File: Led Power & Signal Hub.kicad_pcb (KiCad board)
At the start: 2 copper layers, 3 parts, among them J1 Conn_01x03_Female, J2 Conn_01x04_Female, J3 Conn_01x03_Female

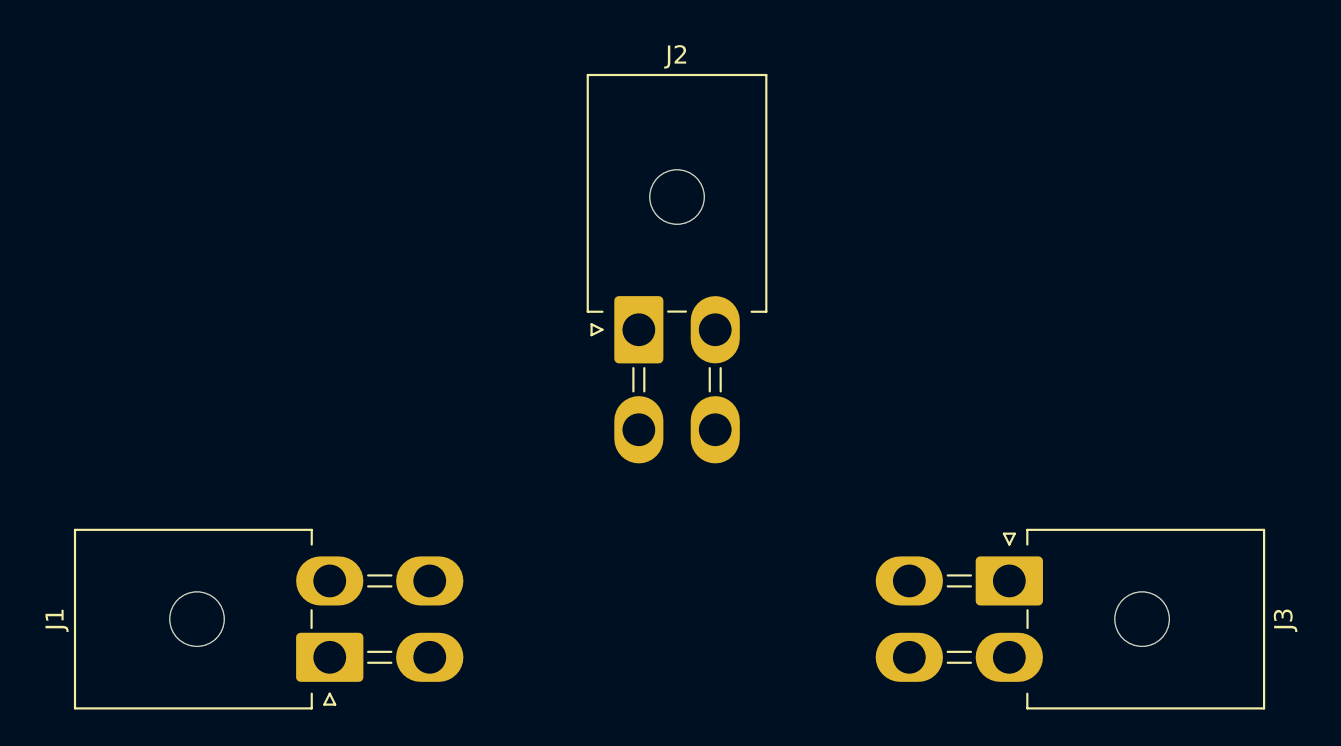
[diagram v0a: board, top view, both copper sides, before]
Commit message: Gotowe PCB
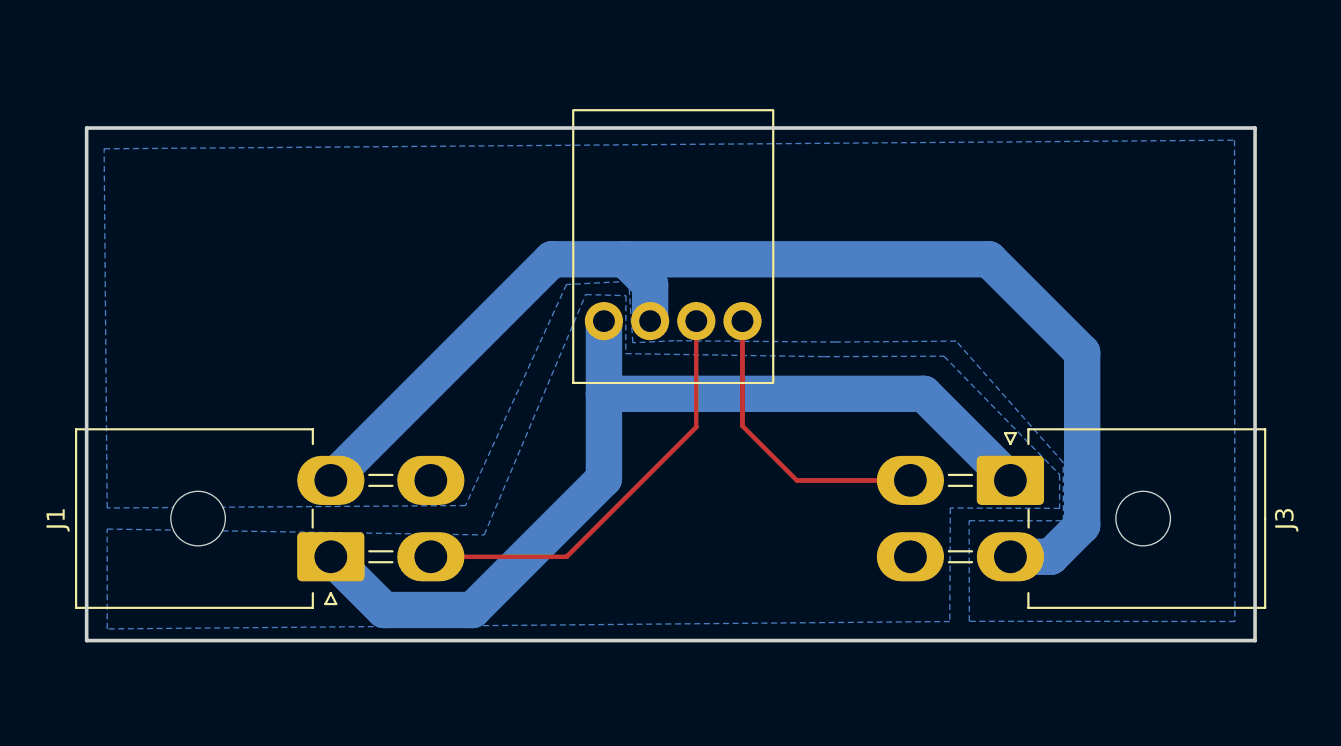
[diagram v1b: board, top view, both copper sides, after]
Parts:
- J2: footprint Connector_Molex:Molex_Mini-Fit_Jr_5569-04A2_2x02_P4.20mm_Horizontal -> SamacSys_Parts:Gniazdo WF kątowe
- moved J1 5.53 mm to (103.8, 96.2)
- moved J3 5.53 mm to (141.1, 92.0)
- moved J2 1.97 mm to (118.8, 83.3)
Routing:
- net Net-(J1-Pad2): track 0.00 -> 66.6 mm
- net Net-(J1-Pad1): track 0.00 -> 52.2 mm
- net Net-(J1-Pad3): track 0.00 -> 23.4 mm
- net Net-(J2-Pad4): track 0.00 -> 16.2 mm
- added copper zone on B.Cu, net Net-(J1-Pad1)
- added copper zone on B.Cu, net Net-(J1-Pad2)
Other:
- board outline added: 64.3 x 28.2 mm
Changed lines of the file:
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@@
   )
   (setup
+    (stackup
+      (layer "F.SilkS" (type "Top Silk Screen"))
+      (layer "F.Paste" (type "Top Solder Paste"))
+      (layer "F.Mask" (type "Top Solder Mask") (thickness 0.01))
+      (layer "F.Cu" (type "copper") (thickness 0.035))
+      (layer "dielectric 1" (type "core") (thickness 1.51) (material "FR4") (epsilon_r 4.5) (loss_tangent 0.02))
+      (layer "B.Cu" (type "copper") (thickness 0.035))
+      (layer "B.Mask" (type "Bottom Solder Mask") (thickness 0.01))
+      (layer "B.Paste" (type "Bottom Solder Paste"))
+      (layer "B.SilkS" (type "Bottom Silk Screen"))
+      (copper_finish "None")
+      (dielectric_constraints no)
+    )
     (pad_to_mask_clearance 0)
     (pcbplotparams
@@
   (net 3 "Net-(J1-Pad3)")
   (net 4 "Net-(J2-Pad4)")
-  (footprint "Connector_Molex:Molex_Mini-Fit_Jr_5569-04A2_2x02_P4.20mm_Horizontal" (layer "F.Cu")
-    (at 120.7 83.765)
-    (descr "Molex Mini-Fit Jr. Power Connectors, old mpn/engineering number: 5569-04A2, example for new mpn: 39-30-0040, 2 Pins per row, Mounting: Snap-in Plastic Peg PCB Lock (http://www.molex.com/pdm_docs/sd/039300020_sd.pdf), generated with kicad-footprint-generator")
-    (tags "connector Molex Mini-Fit_Jr top entryplastic_peg")
+  (footprint "SamacSys_Parts:Gniazdo WF kątowe" (layer "F.Cu")
+    (at 118.79 83.29)
     (property "Sheetfile" "Led Power & Signal Hub.kicad_sch")
     (property "Sheetname" "")
     (attr through_hole)
-    (fp_text reference "J2" (at 2.1 -15.1) (layer "F.SilkS")
-      (effects (font (size 1 1) (thickness 0.15)))
-    )
-    (fp_text value "Conn_01x04_Female" (at 2.1 8.55) (layer "F.Fab")
-      (effects (font (size 1 1) (thickness 0.15)))
-    )
-    (fp_text user "${REFERENCE}" (at 2.1 -13.2) (layer "F.Fab")
-      (effects (font (size 1 1) (thickness 0.15)))
-    )
-    (fp_line (start -2 0) (end -2.6 0.3) (layer "F.SilkS") (width 0.12))
-    (fp_line (start -2 -0.99) (end -2.81 -0.99) (layer "F.SilkS") (width 0.12))
-    (fp_line (start 7.01 -14.01) (end 2.1 -14.01) (layer "F.SilkS") (width 0.12))
-    (fp_line (start 1.61 -1) (end 2.59 -1) (layer "F.SilkS") (width 0.12))
-    (fp_line (start 3.9 2.11) (end 3.9 3.39) (layer "F.SilkS") (width 0.12))
-    (fp_line (start -2.81 -14.01) (end 2.1 -14.01) (layer "F.SilkS") (width 0.12))
-    (fp_line (start -2.81 -0.99) (end -2.81 -14.01) (layer "F.SilkS") (width 0.12))
-    (fp_line (start -2.6 0.3) (end -2.6 -0.3) (layer "F.SilkS") (width 0.12))
-    (fp_line (start -2.6 -0.3) (end -2 0) (layer "F.SilkS") (width 0.12))
-    (fp_line (start 4.5 2.11) (end 4.5 3.39) (layer "F.SilkS") (width 0.12))
-    (fp_line (start -0.3 2.11) (end -0.3 3.39) (layer "F.SilkS") (width 0.12))
-    (fp_line (start 0.3 2.11) (end 0.3 3.39) (layer "F.SilkS") (width 0.12))
-    (fp_line (start 7.01 -0.99) (end 7.01 -14.01) (layer "F.SilkS") (width 0.12))
-    (fp_line (start 6.2 -0.99) (end 7.01 -0.99) (layer "F.SilkS") (width 0.12))
-    (fp_line (start -3.2 -14.4) (end -3.2 7.85) (layer "F.CrtYd") (width 0.05))
-    (fp_line (start 7.4 -14.4) (end -3.2 -14.4) (layer "F.CrtYd") (width 0.05))
-    (fp_line (start 7.4 7.85) (end 7.4 -14.4) (layer "F.CrtYd") (width 0.05))
-    (fp_line (start -3.2 7.85) (end 7.4 7.85) (layer "F.CrtYd") (width 0.05))
-    (fp_line (start -1 -1.1) (end 0 -2.514214) (layer "F.Fab") (width 0.1))
-    (fp_line (start -2.7 -13.9) (end -2.7 -1.1) (layer "F.Fab") (width 0.1))
-    (fp_line (start -2.7 -1.1) (end 6.9 -1.1) (layer "F.Fab") (width 0.1))
-    (fp_line (start 0 -2.514214) (end 1 -1.1) (layer "F.Fab") (width 0.1))
-    (fp_line (start 6.9 -1.1) (end 6.9 -13.9) (layer "F.Fab") (width 0.1))
-    (fp_line (start 6.9 -13.9) (end -2.7 -13.9) (layer "F.Fab") (width 0.1))
-    (pad "" np_thru_hole circle (at 2.1 -7.3) (size 3 3) (drill 3) (layers *.Cu *.Mask))
-    (pad "1" thru_hole roundrect (at 0 0) (size 2.7 3.7) (drill 1.8) (layers *.Cu *.Mask) (roundrect_rratio 0.092593)
+    (fp_text reference "J2" (at 0 -0.5 unlocked) (layer "F.SilkS") hide
+      (effects (font (size 1 1) (thickness 0.15)))
+    )
+    (fp_text value "Conn_01x04_Female" (at 0.1 5.29 unlocked) (layer "F.Fab")
+      (effects (font (size 1 1) (thickness 0.15)))
+    )
+    (fp_text user "${REFERENCE}" (at 0.23 7.23 unlocked) (layer "F.Fab")
+      (effects (font (size 1 1) (thickness 0.15)))
+    )
+    (fp_rect (start -1.7 3.4) (end 9.3 -11.6) (layer "F.SilkS") (width 0.12) (fill none))
+    (pad "1" thru_hole circle (at -0.01 0) (size 2.1 2.1) (drill 1.2) (layers *.Cu *.Mask)
       (net 1 "Net-(J1-Pad1)") (pinfunction "Pin_1") (pintype "passive"))
-    (pad "2" thru_hole oval (at 4.2 0) (size 2.7 3.7) (drill 1.8) (layers *.Cu *.Mask)
+    (pad "2" thru_hole circle (at 2.53 0) (size 2.1 2.1) (drill 1.2) (layers *.Cu *.Mask)
       (net 2 "Net-(J1-Pad2)") (pinfunction "Pin_2") (pintype "passive"))
-    (pad "3" thru_hole oval (at 0 5.5) (size 2.7 3.7) (drill 1.8) (layers *.Cu *.Mask)
+    (pad "3" thru_hole circle (at 5.07 0) (size 2.1 2.1) (drill 1.2) (layers *.Cu *.Mask)
       (net 3 "Net-(J1-Pad3)") (pinfunction "Pin_3") (pintype "passive"))
-    (pad "4" thru_hole oval (at 4.2 5.5) (size 2.7 3.7) (drill 1.8) (layers *.Cu *.Mask)
+    (pad "4" thru_hole circle (at 7.61 0) (size 2.1 2.1) (drill 1.2) (layers *.Cu *.Mask)
       (net 4 "Net-(J2-Pad4)") (pinfunction "Pin_4") (pintype "passive"))
-    (model "${KICAD6_3DMODEL_DIR}/Connector_Molex.3dshapes/Molex_Mini-Fit_Jr_5569-04A2_2x02_P4.20mm_Horizontal.wrl"
-      (offset (xyz 0 0 0))
-      (scale (xyz 1 1 1))
-      (rotate (xyz 0 0 0))
-    )
   )
   (footprint "Connector_Molex:Molex_Mini-Fit_Jr_5569-04A2_2x02_P4.20mm_Horizontal" (layer "F.Cu")
-    (at 103.7 101.78 90)
+    (at 103.76 96.25 90)
     (descr "Molex Mini-Fit Jr. Power Connectors, old mpn/engineering number: 5569-04A2, example for new mpn: 39-30-0040, 2 Pins per row, Mounting: Snap-in Plastic Peg PCB Lock (http://www.molex.com/pdm_docs/sd/039300020_sd.pdf), generated with kicad-footprint-generator")
     (tags "connector Molex Mini-Fit_Jr top entryplastic_peg")
@@
   )
   (footprint "Connector_Molex:Molex_Mini-Fit_Jr_5569-04A2_2x02_P4.20mm_Horizontal" (layer "F.Cu")
-    (at 141.075 97.58 -90)
+    (at 141.135 92.05 -90)
     (descr "Molex Mini-Fit Jr. Power Connectors, old mpn/engineering number: 5569-04A2, example for new mpn: 39-30-0040, 2 Pins per row, Mounting: Snap-in Plastic Peg PCB Lock (http://www.molex.com/pdm_docs/sd/039300020_sd.pdf), generated with kicad-footprint-generator")
     (tags "connector Molex Mini-Fit_Jr top entryplastic_peg")
@@
     )
   )
+  (gr_rect (start 90.33 72.67) (end 154.59 100.86) (layer "Edge.Cuts") (width 0.2) (fill none))
+  (segment (start 118.78 87.29) (end 118.78 83.29) (width 2) (layer "B.Cu") (net 1))
+  (segment (start 103.76 96.25) (end 106.69 99.18) (width 2) (layer "B.Cu") (net 1))
+  (segment (start 136.375 87.29) (end 141.135 92.05) (width 2) (layer "B.Cu") (net 1))
+  (segment (start 106.69 99.18) (end 111.55 99.18) (width 2) (layer "B.Cu") (net 1))
+  (segment (start 118.78 91.95) (end 118.78 87.29) (width 2) (layer "B.Cu") (net 1))
+  (segment (start 118.78 87.29) (end 136.375 87.29) (width 2) (layer "B.Cu") (net 1))
+  (segment (start 111.55 99.18) (end 118.78 91.95) (width 2) (layer "B.Cu") (net 1))
+  (segment (start 119.93 79.89) (end 121.32 81.28) (width 2) (layer "B.Cu") (net 2))
+  (segment (start 143.35 96.25) (end 141.135 96.25) (width 2) (layer "B.Cu") (net 2))
+  (segment (start 121.32 81.28) (end 121.32 83.29) (width 2) (layer "B.Cu") (net 2))
+  (segment (start 103.76 92.05) (end 115.92 79.89) (width 2) (layer "B.Cu") (net 2))
+  (segment (start 119.93 79.89) (end 139.95 79.89) (width 2) (layer "B.Cu") (net 2))
+  (segment (start 115.92 79.89) (end 119.93 79.89) (width 2) (layer "B.Cu") (net 2))
+  (segment (start 145.08 94.52) (end 143.35 96.25) (width 2) (layer "B.Cu") (net 2))
+  (segment (start 145.08 85.02) (end 145.08 94.52) (width 2) (layer "B.Cu") (net 2))
+  (segment (start 139.95 79.89) (end 145.08 85.02) (width 2) (layer "B.Cu") (net 2))
+  (segment (start 116.73 96.25) (end 123.86 89.12) (width 0.25) (layer "F.Cu") (net 3))
+  (segment (start 109.26 96.25) (end 116.73 96.25) (width 0.25) (layer "F.Cu") (net 3))
+  (segment (start 123.86 89.12) (end 123.86 83.29) (width 0.25) (layer "F.Cu") (net 3))
+  (segment (start 126.4 83.29) (end 126.4 89.06) (width 0.25) (layer "F.Cu") (net 4))
+  (segment (start 126.4 89.06) (end 129.39 92.05) (width 0.25) (layer "F.Cu") (net 4))
+  (segment (start 129.39 92.05) (end 135.635 92.05) (width 0.25) (layer "F.Cu") (net 4))
+  (zone (net 1) (net_name "Net-(J1-Pad1)") (layer "B.Cu") (hatch edge 0.508)
+    (connect_pads (clearance 0.508))
+    (min_thickness 0.254) (filled_areas_thickness no)
+    (fill yes (thermal_gap 0.508) (thermal_bridge_width 0.508))
+    (polygon
+      (pts
+        (xy 119.98 85.08)
+        (xy 130.889625 85.244852)
+        (xy 137.48 85.22)
+        (xy 143.84 91.73)
+        (xy 143.84 93.59)
+        (xy 137.83 93.57)
+        (xy 137.8 99.81)
+        (xy 91.46 100.22)
+        (xy 91.458566 94.726438)
+        (xy 112.193588 95.050199)
+        (xy 117.78 81.83)
+        (xy 119.99 81.89)
+      )
+    )
+  )
+  (zone (net 2) (net_name "Net-(J1-Pad2)") (layer "B.Cu") (hatch edge 0.508)
+    (connect_pads (clearance 0.508))
+    (min_thickness 0.254) (filled_areas_thickness no)
+    (fill yes (thermal_gap 0.508) (thermal_bridge_width 0.508))
+    (polygon
+      (pts
+        (xy 153.48 99.81)
+        (xy 138.873667 99.798729)
+        (xy 138.863589 94.268516)
+        (xy 144.049922 94.269787)
+        (xy 144.04 91.07)
+        (xy 138.15 84.39)
+        (xy 131.54 84.44)
+        (xy 122.65 84.37)
+        (xy 120.37 84.48)
+        (xy 120.14 81.1)
+        (xy 116.72 81.28)
+        (xy 111.167716 93.433892)
+        (xy 91.458839 93.567825)
+        (xy 91.291123 73.813933)
+        (xy 153.46 73.34)
+      )
+    )
+  )
